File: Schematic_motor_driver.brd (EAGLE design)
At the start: 50 x 50 mm, 29 parts, among them Q2 IRF540, Q3 IRF540, Q4 IRF540, Q5 IRF540, U1 IR2104PBF, U2 IR2104PBF

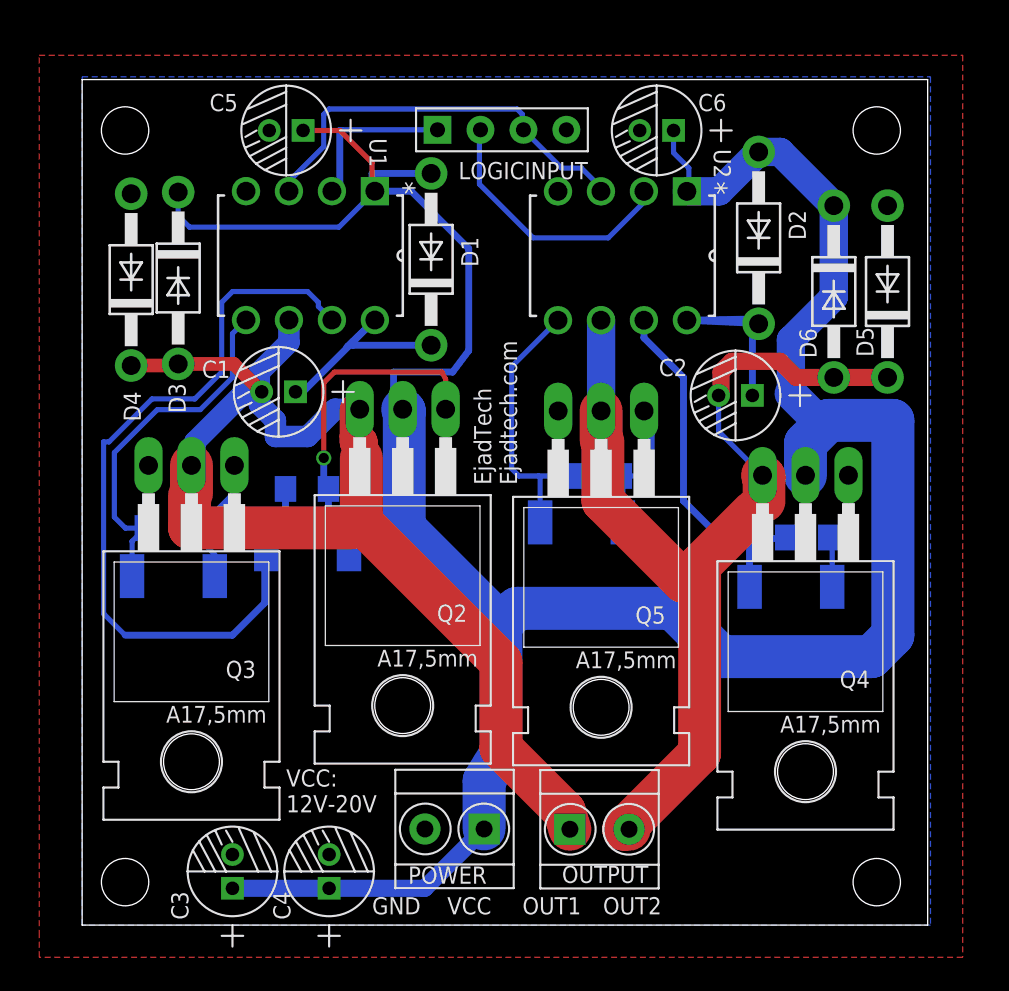
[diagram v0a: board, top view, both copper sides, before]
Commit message: PCB Cosmetics
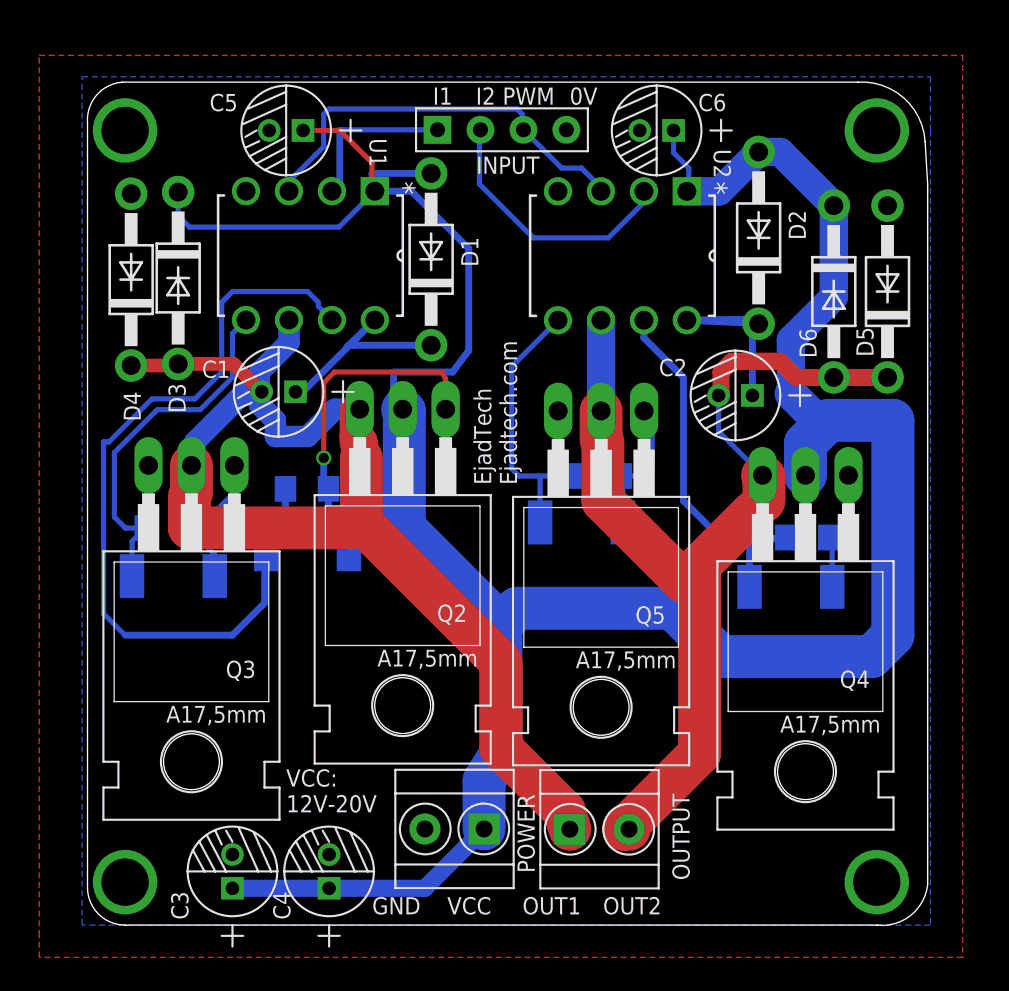
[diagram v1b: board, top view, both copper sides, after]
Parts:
- renumbered LOGICINPUT to INPUT
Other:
- board size 50 x 50 mm -> 49.7 x 49.9 mm
- board text added: "0V"
- board text added: "I1"
- board text added: "I2"
- board text added: "PWM"
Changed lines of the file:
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@@
 <?xml version="1.0" encoding="utf-8"?>
 <!DOCTYPE eagle SYSTEM "eagle.dtd">
-<eagle version="7.6.0">
+<eagle version="7.2.0">
 <drawing>
 <settings>
@@
 <setting verticaltext="up"/>
 </settings>
-<grid distance="0.0125" unitdist="inch" unit="inch" style="lines" multiple="1" display="no" altdistance="0.025" altunitdist="inch" altunit="inch"/>
+<grid distance="0.0125" unitdist="inch" unit="mm" style="lines" multiple="1" display="no" altdistance="0.025" altunitdist="inch" altunit="mm"/>
 <layers>
 <layer number="1" name="Top" color="4" fill="1" visible="yes" active="yes"/>
@@
 <layer number="17" name="Pads" color="2" fill="1" visible="yes" active="yes"/>
 <layer number="18" name="Vias" color="2" fill="1" visible="yes" active="yes"/>
-<layer number="19" name="Unrouted" color="6" fill="1" visible="yes" active="yes"/>
+<layer number="19" name="Unrouted" color="6" fill="1" visible="no" active="yes"/>
 <layer number="20" name="Dimension" color="15" fill="1" visible="yes" active="yes"/>
 <layer number="21" name="tPlace" color="7" fill="1" visible="yes" active="yes"/>
 <layer number="22" name="bPlace" color="7" fill="1" visible="yes" active="yes"/>
-<layer number="23" name="tOrigins" color="15" fill="1" visible="yes" active="yes"/>
-<layer number="24" name="bOrigins" color="15" fill="1" visible="yes" active="yes"/>
+<layer number="23" name="tOrigins" color="15" fill="1" visible="no" active="yes"/>
+<layer number="24" name="bOrigins" color="15" fill="1" visible="no" active="yes"/>
 <layer number="25" name="tNames" color="7" fill="1" visible="yes" active="yes"/>
 <layer number="26" name="bNames" color="7" fill="1" visible="yes" active="yes"/>
@@
 <board>
 <plain>
-<wire x1="0" y1="0" x2="50" y2="0" width="0" layer="20"/>
-<wire x1="50" y1="0" x2="50" y2="50" width="0" layer="20"/>
-<wire x1="50" y1="50" x2="0" y2="50" width="0" layer="20"/>
-<wire x1="0" y1="50" x2="0" y2="0" width="0" layer="20"/>
-<hole x="2.54" y="2.54" drill="2.8"/>
-<hole x="46.99" y="2.54" drill="2.8"/>
-<hole x="46.99" y="46.99" drill="2.8"/>
-<hole x="2.54" y="46.99" drill="2.8"/>
+<wire x1="0.3175" y1="2.2225" x2="2.54" y2="0" width="0" layer="20" curve="90"/>
+<wire x1="2.54" y1="0" x2="46.99" y2="0" width="0" layer="20"/>
+<wire x1="46.99" y1="0" x2="50" y2="2.375" width="0" layer="20" curve="90"/>
+<wire x1="50" y1="2.375" x2="50" y2="43.815" width="0" layer="20"/>
+<wire x1="50" y1="43.815" x2="49.8475" y2="46.3425" width="0" layer="20"/>
+<wire x1="49.8475" y1="46.3425" x2="45.8725" y2="49.8475" width="0" layer="20" curve="90"/>
+<wire x1="45.8725" y1="49.8475" x2="2.3875" y2="49.8475" width="0" layer="20"/>
+<wire x1="2.3875" y1="49.8475" x2="0.3175" y2="47.46" width="0" layer="20" curve="90"/>
+<wire x1="0.3175" y1="47.46" x2="0.3175" y2="2.2225" width="0" layer="20"/>
 <text x="26.035" y="0.635" size="1.016" layer="25" font="vector" ratio="12">OUT1</text>
 <text x="30.7975" y="0.635" size="1.016" layer="25" font="vector" ratio="12">OUT2</text>
@@
 <text x="25.7175" y="26.035" size="1.016" layer="25" font="vector" ratio="12" rot="R90">EjadTech
 Ejadtech.com</text>
+<text x="30.48" y="49.53" size="1.016" layer="25" font="vector" ratio="12" rot="R180">0V</text>
+<text x="21.9075" y="49.53" size="1.016" layer="25" font="vector" ratio="12" rot="R180">I1</text>
+<text x="24.4475" y="49.53" size="1.016" layer="25" font="vector" ratio="12" rot="R180">I2</text>
+<text x="27.94" y="49.53" size="1.016" layer="25" font="vector" ratio="12" rot="R180">PWM</text>
 </plain>
 <attributes>
@@
 <attribute name="VALUE" x="50.419" y="35.433" size="1.27" layer="27" ratio="10" rot="R90"/>
 </element>
-<element name="LOGICINPUT" library="Seeed-Connector -2016" package="H4-2.54" value="4p-2.54" x="24.825" y="47.03" smashed="yes" rot="R90">
+<element name="INPUT" library="Seeed-Connector -2016" package="H4-2.54" value="4p-2.54" x="24.825" y="47.03" smashed="yes" rot="R90">
 <attribute name="MPN" value="F185-1104A1BSYA1" x="24.825" y="47.03" size="1.778" layer="27" rot="R90" display="off"/>
-<attribute name="NAME" x="29.905" y="45.125" size="1.016" layer="25" font="vector" ratio="12" rot="R180"/>
+<attribute name="NAME" x="27.0475" y="45.4425" size="1.016" layer="25" font="vector" ratio="12" rot="R180"/>
 <attribute name="VALUE" x="26.73" y="49.57" size="0.889" layer="27" ratio="11" rot="R180"/>
 </element>
 <element name="OUTPUT" library="Seeed-Connector -2016" package="H2-3.5-7.0X7.0MM" value="GREEN-2P-3.5" x="30.5925" y="5.6675" smashed="yes">
-<attribute name="NAME" x="28.37" y="2.4925" size="1.016" layer="25" font="vector" ratio="12"/>
+<attribute name="NAME" x="35.925" y="2.6525" size="1.016" layer="25" font="vector" ratio="12" rot="R90"/>
 <attribute name="VALUE" x="28.6875" y="1.2225" size="0.889" layer="27" ratio="11"/>
 </element>
 <element name="POWER" library="Seeed-Connector -2016" package="H2-3.5-7.0X7.0MM" value="GREEN-2P-3.5" x="22.02" y="5.685" smashed="yes" rot="R180">
-<attribute name="NAME" x="23.925" y="3.4625" size="1.016" layer="25" font="vector" ratio="12" rot="R180"/>
+<attribute name="NAME" x="25.7475" y="7.7325" size="1.016" layer="25" font="vector" ratio="12" rot="R270"/>
 <attribute name="VALUE" x="23.925" y="10.13" size="0.889" layer="27" ratio="11" rot="R180"/>
 </element>
@@
 <signals>
 <signal name="IN1">
-<contactref element="LOGICINPUT" pad="1"/>
+<contactref element="INPUT" pad="1"/>
 <contactref element="U1" pad="2"/>
 <wire x1="15.3" y1="46.93" x2="15.24" y2="46.99" width="0.4064" layer="16"/>
@@
 </signal>
 <signal name="IN2">
-<contactref element="LOGICINPUT" pad="2"/>
+<contactref element="INPUT" pad="2"/>
 <contactref element="U2" pad="2"/>
 <wire x1="33.22" y1="43.39" x2="33.22" y2="42.745" width="0.3048" layer="16"/>
@@
 </signal>
 <signal name="PWM">
-<contactref element="LOGICINPUT" pad="3"/>
+<contactref element="INPUT" pad="3"/>
 <contactref element="U1" pad="3"/>
 <contactref element="U2" pad="3"/>
@@
 </signal>
 <signal name="GND">
-<contactref element="LOGICINPUT" pad="4"/>
+<contactref element="INPUT" pad="4"/>
 <contactref element="POWER" pad="2"/>
 <contactref element="U2" pad="4"/>
@@
 <wire x1="7.8425" y1="21.91" x2="6.275" y2="23.4775" width="0.3048" layer="16"/>
 </signal>
+<signal name="N$11">
+<via x="2.54" y="46.99" extent="1-16" drill="2.8"/>
+<via x="2.54" y="2.54" extent="1-16" drill="2.8"/>
+<via x="46.99" y="2.54" extent="1-16" drill="2.8"/>
+<via x="46.99" y="46.99" extent="1-16" drill="2.8"/>
+<wire x1="2.54" y1="46.99" x2="46.99" y2="46.99" width="0" layer="19" extent="1-1"/>
+<wire x1="46.99" y1="2.54" x2="46.99" y2="46.99" width="0" layer="19" extent="1-1"/>
+<wire x1="2.54" y1="2.54" x2="2.54" y2="46.99" width="0" layer="19" extent="1-1"/>
+</signal>
 </signals>

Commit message: Revert "PCB Cosmetics"
This reverts commit 40f95e063b70cdd7ef0c66ddfb49b8478f35fe8d.
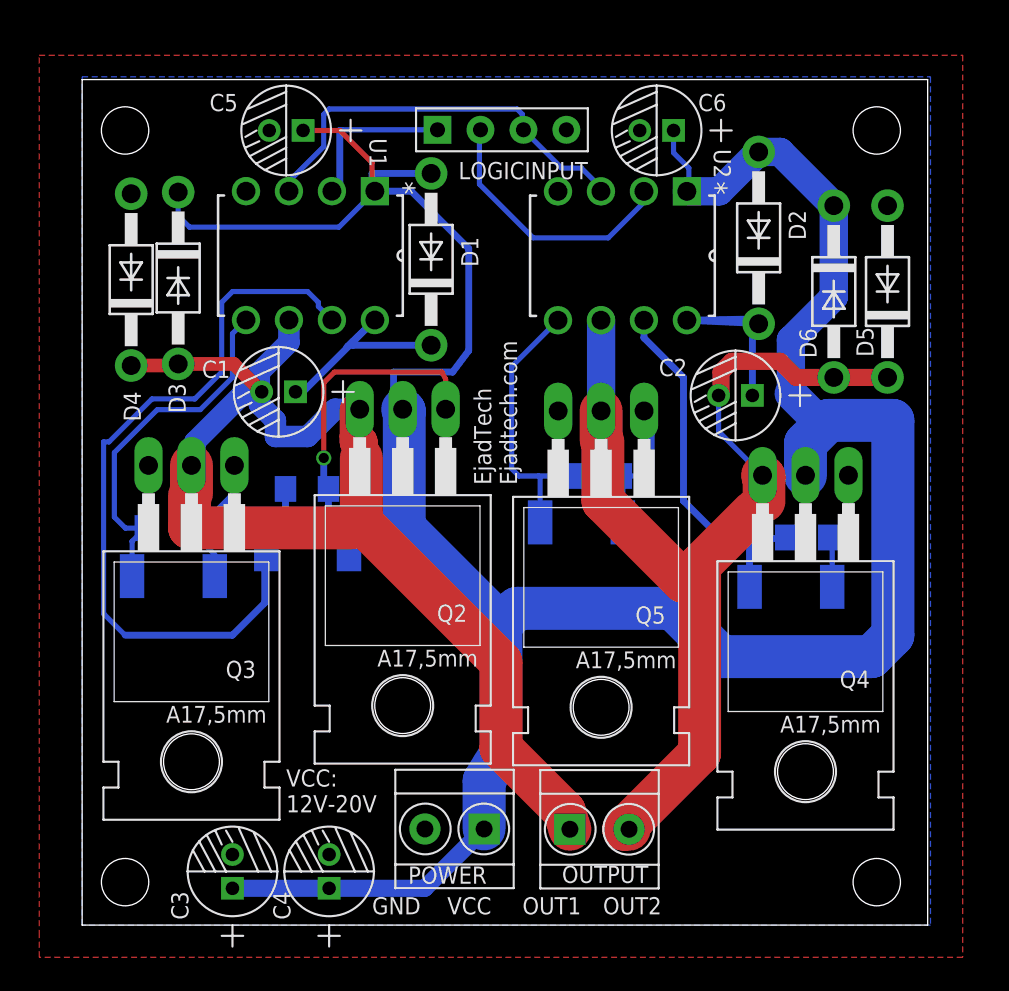
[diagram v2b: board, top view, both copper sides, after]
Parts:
- renumbered INPUT to LOGICINPUT
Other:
- board size 49.7 x 49.9 mm -> 50 x 50 mm
- board text removed: "0V"
- board text removed: "I1"
- board text removed: "I2"
- board text removed: "PWM"
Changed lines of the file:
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@@
 <?xml version="1.0" encoding="utf-8"?>
 <!DOCTYPE eagle SYSTEM "eagle.dtd">
-<eagle version="7.2.0">
+<eagle version="7.6.0">
 <drawing>
 <settings>
@@
 <setting verticaltext="up"/>
 </settings>
-<grid distance="0.0125" unitdist="inch" unit="mm" style="lines" multiple="1" display="no" altdistance="0.025" altunitdist="inch" altunit="mm"/>
+<grid distance="0.0125" unitdist="inch" unit="inch" style="lines" multiple="1" display="no" altdistance="0.025" altunitdist="inch" altunit="inch"/>
 <layers>
 <layer number="1" name="Top" color="4" fill="1" visible="yes" active="yes"/>
@@
 <layer number="17" name="Pads" color="2" fill="1" visible="yes" active="yes"/>
 <layer number="18" name="Vias" color="2" fill="1" visible="yes" active="yes"/>
-<layer number="19" name="Unrouted" color="6" fill="1" visible="no" active="yes"/>
+<layer number="19" name="Unrouted" color="6" fill="1" visible="yes" active="yes"/>
 <layer number="20" name="Dimension" color="15" fill="1" visible="yes" active="yes"/>
 <layer number="21" name="tPlace" color="7" fill="1" visible="yes" active="yes"/>
 <layer number="22" name="bPlace" color="7" fill="1" visible="yes" active="yes"/>
-<layer number="23" name="tOrigins" color="15" fill="1" visible="no" active="yes"/>
-<layer number="24" name="bOrigins" color="15" fill="1" visible="no" active="yes"/>
+<layer number="23" name="tOrigins" color="15" fill="1" visible="yes" active="yes"/>
+<layer number="24" name="bOrigins" color="15" fill="1" visible="yes" active="yes"/>
 <layer number="25" name="tNames" color="7" fill="1" visible="yes" active="yes"/>
 <layer number="26" name="bNames" color="7" fill="1" visible="yes" active="yes"/>
@@
 <board>
 <plain>
-<wire x1="0.3175" y1="2.2225" x2="2.54" y2="0" width="0" layer="20" curve="90"/>
-<wire x1="2.54" y1="0" x2="46.99" y2="0" width="0" layer="20"/>
-<wire x1="46.99" y1="0" x2="50" y2="2.375" width="0" layer="20" curve="90"/>
-<wire x1="50" y1="2.375" x2="50" y2="43.815" width="0" layer="20"/>
-<wire x1="50" y1="43.815" x2="49.8475" y2="46.3425" width="0" layer="20"/>
-<wire x1="49.8475" y1="46.3425" x2="45.8725" y2="49.8475" width="0" layer="20" curve="90"/>
-<wire x1="45.8725" y1="49.8475" x2="2.3875" y2="49.8475" width="0" layer="20"/>
-<wire x1="2.3875" y1="49.8475" x2="0.3175" y2="47.46" width="0" layer="20" curve="90"/>
-<wire x1="0.3175" y1="47.46" x2="0.3175" y2="2.2225" width="0" layer="20"/>
+<wire x1="0" y1="0" x2="50" y2="0" width="0" layer="20"/>
+<wire x1="50" y1="0" x2="50" y2="50" width="0" layer="20"/>
+<wire x1="50" y1="50" x2="0" y2="50" width="0" layer="20"/>
+<wire x1="0" y1="50" x2="0" y2="0" width="0" layer="20"/>
+<hole x="2.54" y="2.54" drill="2.8"/>
+<hole x="46.99" y="2.54" drill="2.8"/>
+<hole x="46.99" y="46.99" drill="2.8"/>
+<hole x="2.54" y="46.99" drill="2.8"/>
 <text x="26.035" y="0.635" size="1.016" layer="25" font="vector" ratio="12">OUT1</text>
 <text x="30.7975" y="0.635" size="1.016" layer="25" font="vector" ratio="12">OUT2</text>
@@
 <text x="25.7175" y="26.035" size="1.016" layer="25" font="vector" ratio="12" rot="R90">EjadTech
 Ejadtech.com</text>
-<text x="30.48" y="49.53" size="1.016" layer="25" font="vector" ratio="12" rot="R180">0V</text>
-<text x="21.9075" y="49.53" size="1.016" layer="25" font="vector" ratio="12" rot="R180">I1</text>
-<text x="24.4475" y="49.53" size="1.016" layer="25" font="vector" ratio="12" rot="R180">I2</text>
-<text x="27.94" y="49.53" size="1.016" layer="25" font="vector" ratio="12" rot="R180">PWM</text>
 </plain>
 <attributes>
@@
 <attribute name="VALUE" x="50.419" y="35.433" size="1.27" layer="27" ratio="10" rot="R90"/>
 </element>
-<element name="INPUT" library="Seeed-Connector -2016" package="H4-2.54" value="4p-2.54" x="24.825" y="47.03" smashed="yes" rot="R90">
+<element name="LOGICINPUT" library="Seeed-Connector -2016" package="H4-2.54" value="4p-2.54" x="24.825" y="47.03" smashed="yes" rot="R90">
 <attribute name="MPN" value="F185-1104A1BSYA1" x="24.825" y="47.03" size="1.778" layer="27" rot="R90" display="off"/>
-<attribute name="NAME" x="27.0475" y="45.4425" size="1.016" layer="25" font="vector" ratio="12" rot="R180"/>
+<attribute name="NAME" x="29.905" y="45.125" size="1.016" layer="25" font="vector" ratio="12" rot="R180"/>
 <attribute name="VALUE" x="26.73" y="49.57" size="0.889" layer="27" ratio="11" rot="R180"/>
 </element>
 <element name="OUTPUT" library="Seeed-Connector -2016" package="H2-3.5-7.0X7.0MM" value="GREEN-2P-3.5" x="30.5925" y="5.6675" smashed="yes">
-<attribute name="NAME" x="35.925" y="2.6525" size="1.016" layer="25" font="vector" ratio="12" rot="R90"/>
+<attribute name="NAME" x="28.37" y="2.4925" size="1.016" layer="25" font="vector" ratio="12"/>
 <attribute name="VALUE" x="28.6875" y="1.2225" size="0.889" layer="27" ratio="11"/>
 </element>
 <element name="POWER" library="Seeed-Connector -2016" package="H2-3.5-7.0X7.0MM" value="GREEN-2P-3.5" x="22.02" y="5.685" smashed="yes" rot="R180">
-<attribute name="NAME" x="25.7475" y="7.7325" size="1.016" layer="25" font="vector" ratio="12" rot="R270"/>
+<attribute name="NAME" x="23.925" y="3.4625" size="1.016" layer="25" font="vector" ratio="12" rot="R180"/>
 <attribute name="VALUE" x="23.925" y="10.13" size="0.889" layer="27" ratio="11" rot="R180"/>
 </element>
@@
 <signals>
 <signal name="IN1">
-<contactref element="INPUT" pad="1"/>
+<contactref element="LOGICINPUT" pad="1"/>
 <contactref element="U1" pad="2"/>
 <wire x1="15.3" y1="46.93" x2="15.24" y2="46.99" width="0.4064" layer="16"/>
@@
 </signal>
 <signal name="IN2">
-<contactref element="INPUT" pad="2"/>
+<contactref element="LOGICINPUT" pad="2"/>
 <contactref element="U2" pad="2"/>
 <wire x1="33.22" y1="43.39" x2="33.22" y2="42.745" width="0.3048" layer="16"/>
@@
 </signal>
 <signal name="PWM">
-<contactref element="INPUT" pad="3"/>
+<contactref element="LOGICINPUT" pad="3"/>
 <contactref element="U1" pad="3"/>
 <contactref element="U2" pad="3"/>
@@
 </signal>
 <signal name="GND">
-<contactref element="INPUT" pad="4"/>
+<contactref element="LOGICINPUT" pad="4"/>
 <contactref element="POWER" pad="2"/>
 <contactref element="U2" pad="4"/>
@@
 <wire x1="7.8425" y1="21.91" x2="6.275" y2="23.4775" width="0.3048" layer="16"/>
 </signal>
-<signal name="N$11">
-<via x="2.54" y="46.99" extent="1-16" drill="2.8"/>
-<via x="2.54" y="2.54" extent="1-16" drill="2.8"/>
-<via x="46.99" y="2.54" extent="1-16" drill="2.8"/>
-<via x="46.99" y="46.99" extent="1-16" drill="2.8"/>
-<wire x1="2.54" y1="46.99" x2="46.99" y2="46.99" width="0" layer="19" extent="1-1"/>
-<wire x1="46.99" y1="2.54" x2="46.99" y2="46.99" width="0" layer="19" extent="1-1"/>
-<wire x1="2.54" y1="2.54" x2="2.54" y2="46.99" width="0" layer="19" extent="1-1"/>
-</signal>
 </signals>
